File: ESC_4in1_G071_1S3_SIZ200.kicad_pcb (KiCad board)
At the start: 4 copper layers, 28 x 28 mm, 180 parts, among them J1 Conn_01x10, U1 STM32G071GBU6, U10 NCP81161MNTBG, U11 SIZ200DT-T1-GE3, U12 NCP81161MNTBG, U13 SIZ200DT-T1-GE3, U14 TPS630701, U15 TPS72733DSE, U16 INA186A2, U17 STM32G071GBU6, U18 NCP81161MNTBG, U19 SIZ200DT-T1-GE3, U2 NCP81161MNTBG, U20 NCP81161MNTBG, U21 STM32G071GBU6, U22 SIZ200DT-T1-GE3, U23 NCP81161MNTBG, U24 SIZ200DT-T1-GE3, U25 NCP81161MNTBG, U26 SIZ200DT-T1-GE3, U27 NCP81161MNTBG, U28 STM32G071GBU6, U29 SIZ200DT-T1-GE3, U3 SIZ200DT-T1-GE3, U30 NCP81161MNTBG, U31 SIZ200DT-T1-GE3, U4 NCP81161MNTBG, U5 SIZ200DT-T1-GE3, U6 NCP81161MNTBG, U7 SIZ200DT-T1-GE3, U8 NCP81161MNTBG, U9 SIZ200DT-T1-GE3

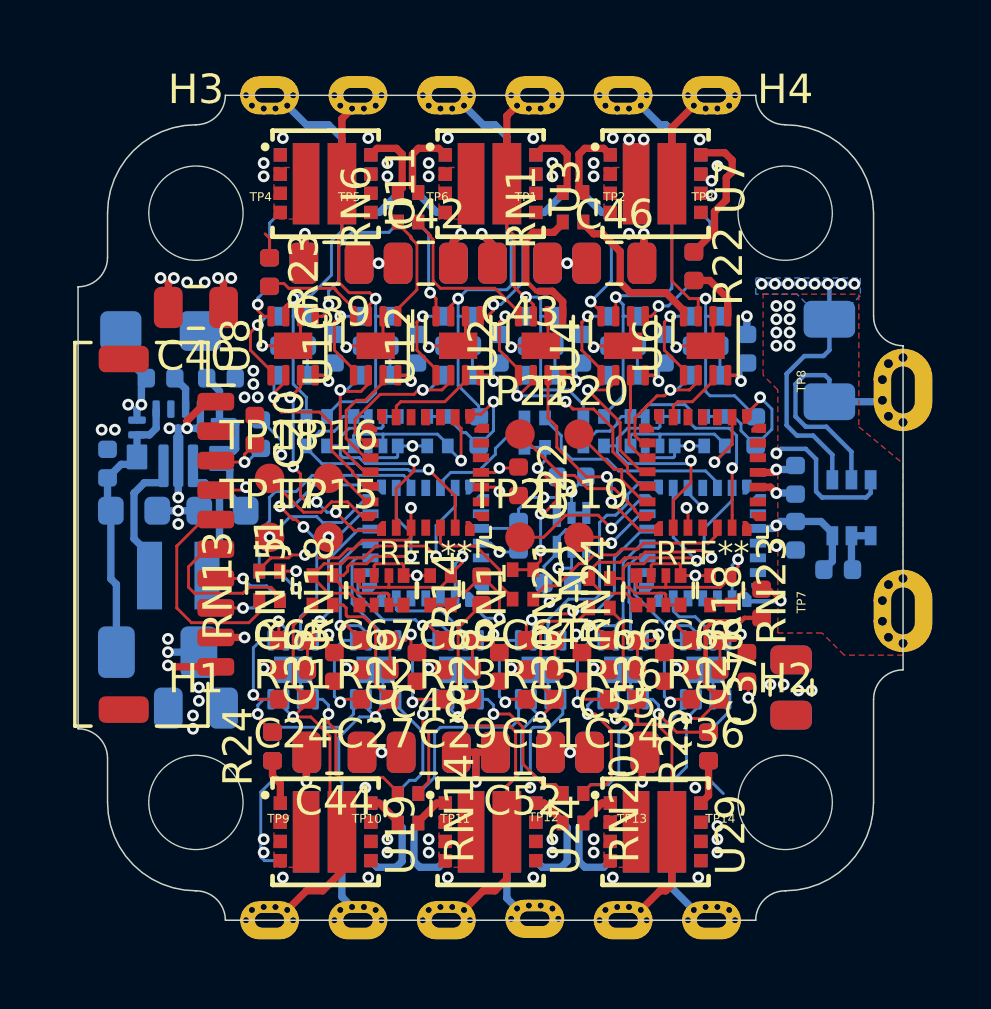
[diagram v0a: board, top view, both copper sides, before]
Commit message: update layout
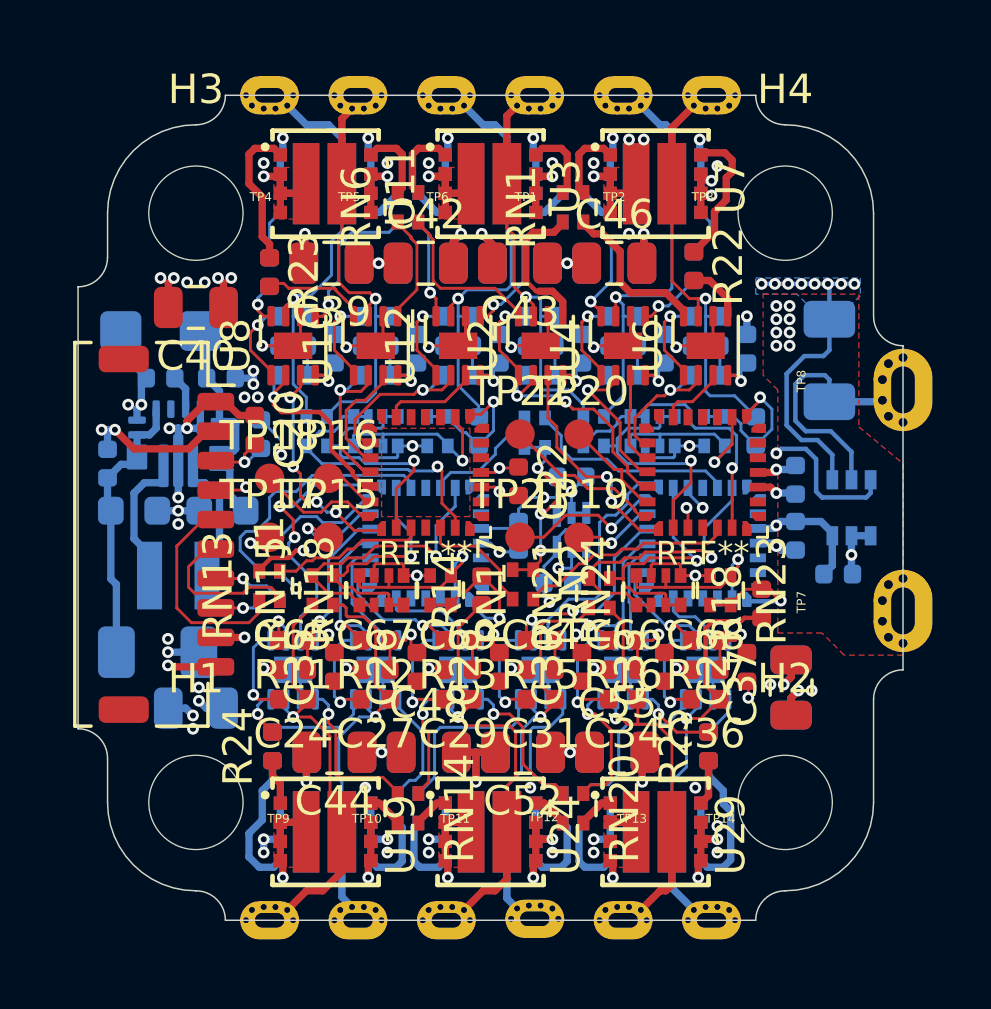
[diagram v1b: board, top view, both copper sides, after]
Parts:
- moved C63 0.15 mm to (147.8, 77.2)
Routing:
- net +BATT: track 18.4 -> 61.3 mm, vias 44 -> 45
- net GND: track 97.2 -> 128.0 mm, vias 76 -> 77
- net /ESC2_IN: track 11.1 -> 5.25 mm, vias 2 -> 0
- net /ESC2_B_GH: track 0.88 -> 5.05 mm
- net /ESC3_C_GL: track 1.32 -> 4.89 mm
- net Net-(C15-Pad2): track 5.83 -> 7.52 mm
- net /ESC4_SWDIO: track 1.76 -> 3.32 mm
- net /ESC4_SWDCLK: track 4.03 -> 5.49 mm
- net +5V: track 40.9 -> 41.7 mm
- net /ESC4_B_GH: track 4.15 -> 4.90 mm, vias 1 -> 0
- net /ESC4_IN: track 8.08 -> 8.78 mm
- net /ESC3_MC: track 3.41 -> 3.97 mm
- added copper zone on F.Cu, net GND

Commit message: update schematic, layout and schematic pdf
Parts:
- L1: value 1u -> 820 nH
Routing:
- added copper zone on In1.Cu_(power), net /ESC3_B
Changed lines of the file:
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@@
       (effects (font (size 1 1) (thickness 0.15)) (justify mirror))
     )
-    (fp_text value 1u (at 0 -2.65) (layer B.Fab)
+    (fp_text value "820 nH" (at 0 -2.65) (layer B.Fab)
       (effects (font (size 1 1) (thickness 0.15)) (justify mirror))
     )
@@
     (polygon
       (pts
-        (xy 150 89) (xy 122 89) (xy 122 61) (xy 150 61)
+        (xy 150 89.5) (xy 122 89.5) (xy 122 61) (xy 150 61)
       )
     )
@@
     (polygon
       (pts
-        (xy 150 89) (xy 122 89) (xy 122 80.5) (xy 144.5 80.5) (xy 145 80)
+        (xy 150 89.5) (xy 122 89.5) (xy 122 80.5) (xy 144.5 80.5) (xy 145 80)
         (xy 145 76.5) (xy 145.5 76) (xy 145.5 74) (xy 145 73.5) (xy 145 70)
         (xy 144.5 69.5) (xy 127 69.5) (xy 123 73.5) (xy 122 73.5) (xy 122 61)
@@
       )
     )
+  )
+  (zone (net 82) (net_name /ESC3_B) (layer "In1.Cu_(power)") (hatch edge 0.508)
+    (connect_pads yes (clearance 0.125))
+    (min_thickness 0.125)
+    (fill yes (arc_segments 32) (thermal_gap 0.508) (thermal_bridge_width 0.508))
+    (polygon
+      (pts
+        (xy 141.75 89.75) (xy 139.25 89.75) (xy 139.25 88.25) (xy 141.75 88.25)
+      )
+    )

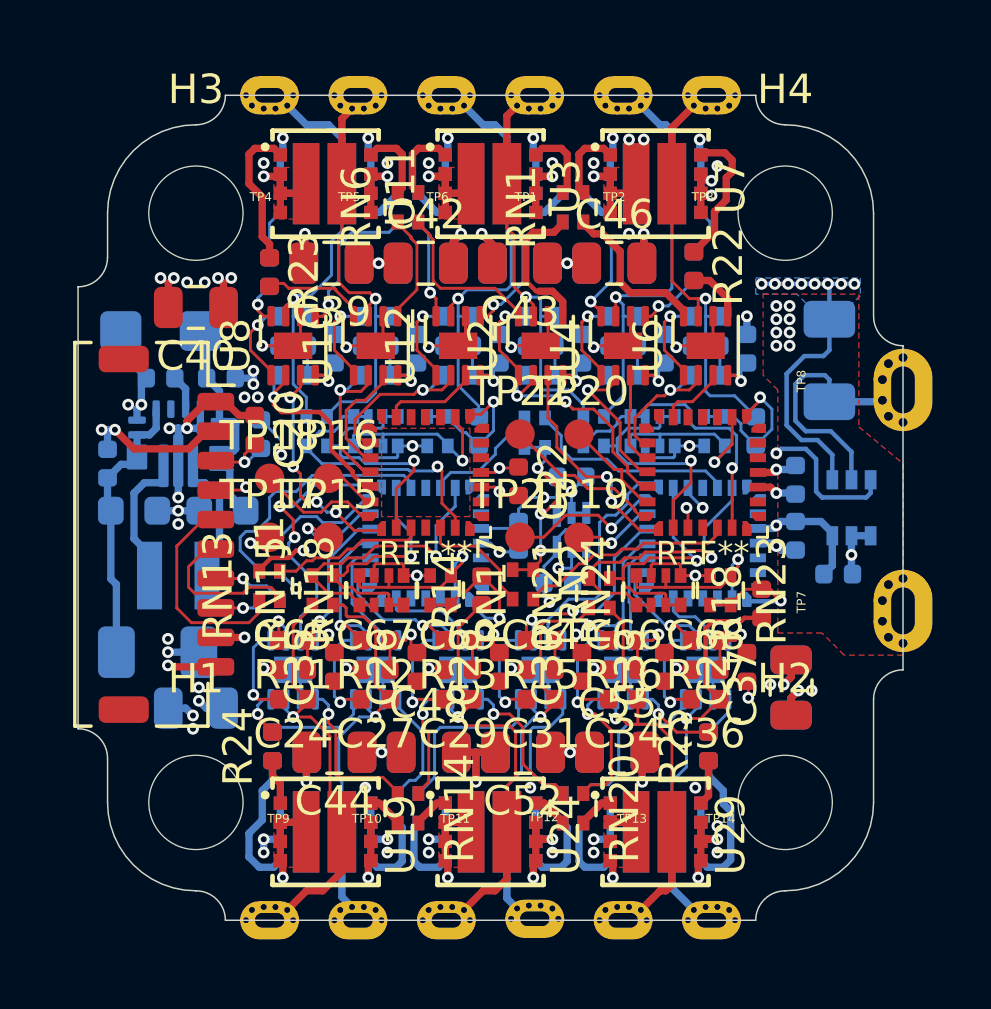
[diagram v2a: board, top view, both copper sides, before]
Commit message: cosmetic update
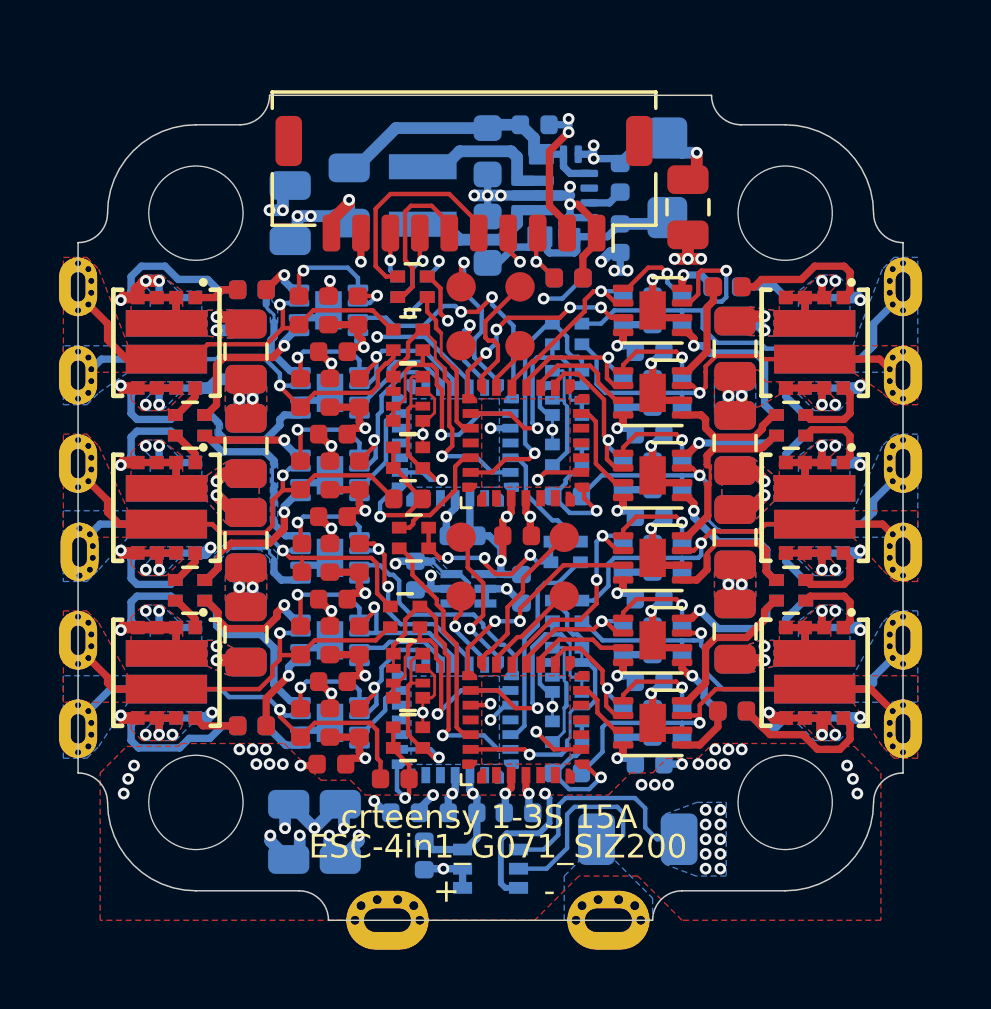
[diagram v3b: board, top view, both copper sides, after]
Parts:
- added C70: 10u, Capacitor_SMD:C_0402_1005Metric, B.Cu at (133.1, 85.3)
- C13: footprint 11_PSoC_FC_whoop:C_1206_3216Metric_dense -> 11_PSoC_FC_whoop:C_0805_2012Metric_dense
- C37: moved to B.Cu
- moved TP14 22.5 mm to (122.0, 82.5), turned to 270 degrees
- moved TP3 22.5 mm to (150.0, 82.5), turned to 90 degrees
- moved TP4 22.5 mm to (150.0, 67.5), turned to 90 degrees
- moved TP9 22.5 mm to (122.0, 67.5), turned to 270 degrees
- moved TP10 20.8 mm to (122.0, 70.5), turned to 270 degrees
- moved TP2 20.8 mm to (150.0, 79.5), turned to 90 degrees
- moved TP13 20.8 mm to (122.0, 79.5), turned to 270 degrees
- moved TP5 20.8 mm to (150.0, 70.5), turned to 90 degrees
- moved TP8 20.6 mm to (140.0, 89.0), turned to 0 degrees
- moved TP7 20.4 mm to (132.5, 89.0), turned to 0 degrees
- moved H1 20.0 mm to (126.0, 65.0), turned to 270 degrees
- moved H2 20.0 mm to (126.0, 85.0), turned to 270 degrees
- moved H3 20.0 mm to (146.0, 65.0), turned to 270 degrees
- moved H4 20.0 mm to (146.0, 85.0), turned to 270 degrees
- moved TP1 19.9 mm to (150.0, 76.5), turned to 90 degrees
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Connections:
- net Net-(R1-Pad2) renamed /Batt-
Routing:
- net GND: track 128.0 -> 135.6 mm, vias 77 -> 80
- net +BATT: track 61.3 -> 67.6 mm, vias 45 -> 62
- net +3V3: track 21.5 -> 17.8 mm, vias 4 -> 5
- net /ESC2_A: track 14.1 -> 17.7 mm
- net /Batt-: track 8.44 -> 6.89 mm
- net +5V: track 41.7 -> 43.1 mm, vias 18 -> 17
- net /ESCx_tele: track 18.0 -> 19.0 mm
- net /ESC1_B_PWM: track 5.93 -> 4.98 mm
- net Net-(R2-Pad2): track 25.1 -> 25.8 mm
- net /ESC2_A_PWM: track 6.99 -> 6.45 mm
- net /ESC4_IN: track 8.78 -> 9.22 mm, vias 0 -> 2
- added copper zone on B.Cu, net +5V
- added copper zone on B.Cu, net +BATT
- added copper zone on B.Cu, net /Batt-
- added copper zone on F.Cu, net /ESC1_A
- added copper zone on F.Cu, net /ESC1_A_DRVH
- added copper zone on B.Cu, net /ESC1_B
- added copper zone on F.Cu, net /ESC1_C
- added copper zone on B.Cu, net /ESC2_A
- added copper zone on F.Cu, net /ESC2_B
- added copper zone on B.Cu, net /ESC2_C
- added copper zone on B.Cu, net /ESC3_A
- added copper zone on B.Cu, net /ESC3_A_DRVH
- added copper zone on B.Cu, net /ESC3_A_DRVL
- added copper zone on F.Cu, net /ESC3_B
- added copper zone on B.Cu, net /ESC3_C
- added copper zone on F.Cu, net /ESC4_A
- added copper zone on B.Cu, net /ESC4_B
- added copper zone on B.Cu, net /ESC4_B_DRVH
- added copper zone on B.Cu, net /ESC4_B_DRVL
- added copper zone on F.Cu, net /ESC4_C
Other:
- outline, holes or cut-outs redrawn
- rule solder_mask_min_width: 0.05 -> 0.1
- board text added: "+"
- board text added: "-"
- board text added: "ESC-4in1_G071_SIZ200"
- board text added: "Gnd VBat Ibat Tele ESC1 ESC2 ESC3 ESC4 5V Gnd"
- board text added: "crteensy 1-3S 15A"
